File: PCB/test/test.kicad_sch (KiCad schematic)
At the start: 57 parts, among them U1 STM32WBxx_QFN48, U2 USBLC6-2SC6, U3 LD3985M33R, X1 NX2016_32MHz, X2 NX2012_32K768Hz

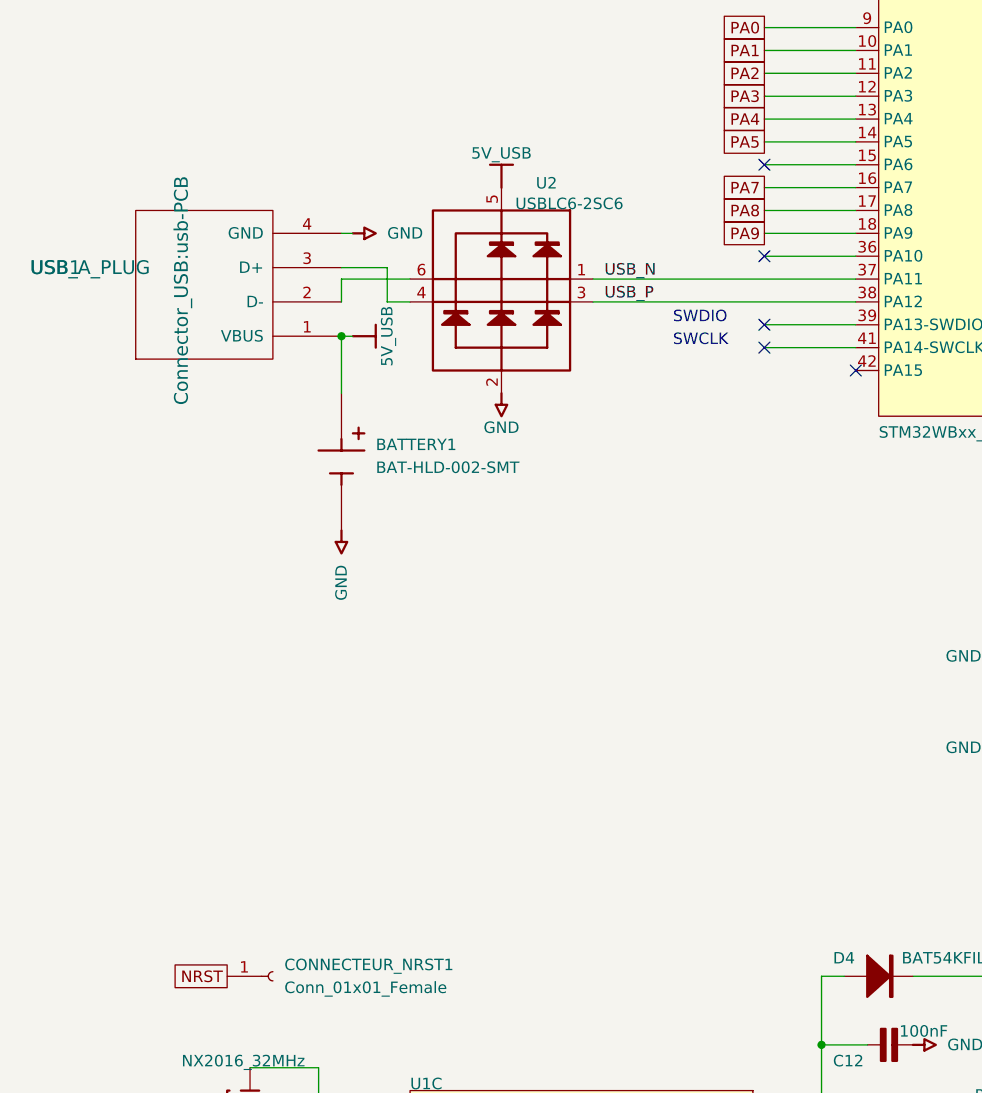
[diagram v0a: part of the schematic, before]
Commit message: ajout headers, reste circuit + UVNC
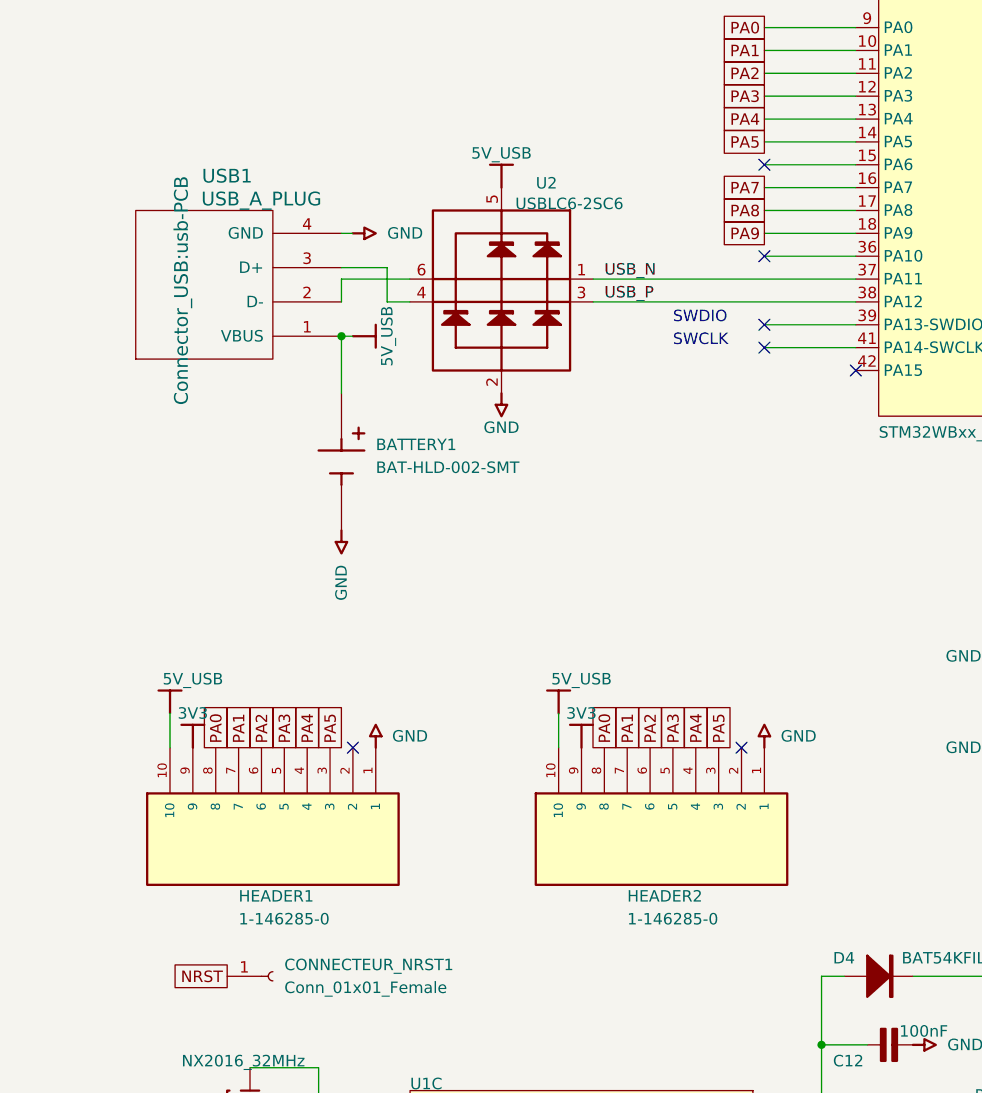
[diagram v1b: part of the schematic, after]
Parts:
- added HEADER1, HEADER2: 1-146285-0, TE_1-146285-0, symbol 1-146285-0:1-146285-0
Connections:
- net 3V3: now also HEADER1.9, HEADER2.9
- net 5V_USB: now also HEADER1.10, HEADER2.10
- net GND: now also HEADER1.1, HEADER2.1
- net PA0: now also HEADER1.8, HEADER2.8
- net PA1: now also HEADER1.7, HEADER2.7
- net PA2: now also HEADER1.6, HEADER2.6
- net PA3: now also HEADER1.5, HEADER2.5
- net PA4: now also HEADER1.4, HEADER2.4
- net PA5: now also HEADER1.3, HEADER2.3
- no-connect marks 14 -> 16
